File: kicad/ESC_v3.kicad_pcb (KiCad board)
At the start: 6 copper layers, 50 x 50 mm, 165 parts, among them J1 Conn_01x05_Pin, J2 Conn_01x05_Pin, J4 Conn_01x06_Pin, J6 Conn_01x06_Pin, J7 Conn_01x02_Pin, J8 Conn_01x04_Pin, J9 Conn_01x02_Pin, Q1 RH6L040BGTB1, Q10 RH6L040BGTB1, Q11 RH6L040BGTB1, Q12 RH6L040BGTB1, Q2 RH6L040BGTB1, Q3 RH6L040BGTB1, Q4 RH6L040BGTB1, Q5 RH6L040BGTB1, Q6 RH6L040BGTB1, Q7 RH6L040BGTB1, Q8 RH6L040BGTB1, Q9 RH6L040BGTB1, SW2 SW_Nidec_CAS-120A1, U1 L6387, U10 BD4104, U11 AMS1117-5.0, U12 ACS711xEXLT-15AB, U13 LM2937xMP, U14 MCP9700x-ETT, U15 MAX40200AUK, U16 AS5048A, U19 STM32G431CBUx, U2 L6387, U3 L6387, U4 L6387, U5 L6387, U6 L6387, U7 AMS1117-3.3, U8 ACS711xEXLT-15AB, U9 ACS711xEXLT-15AB

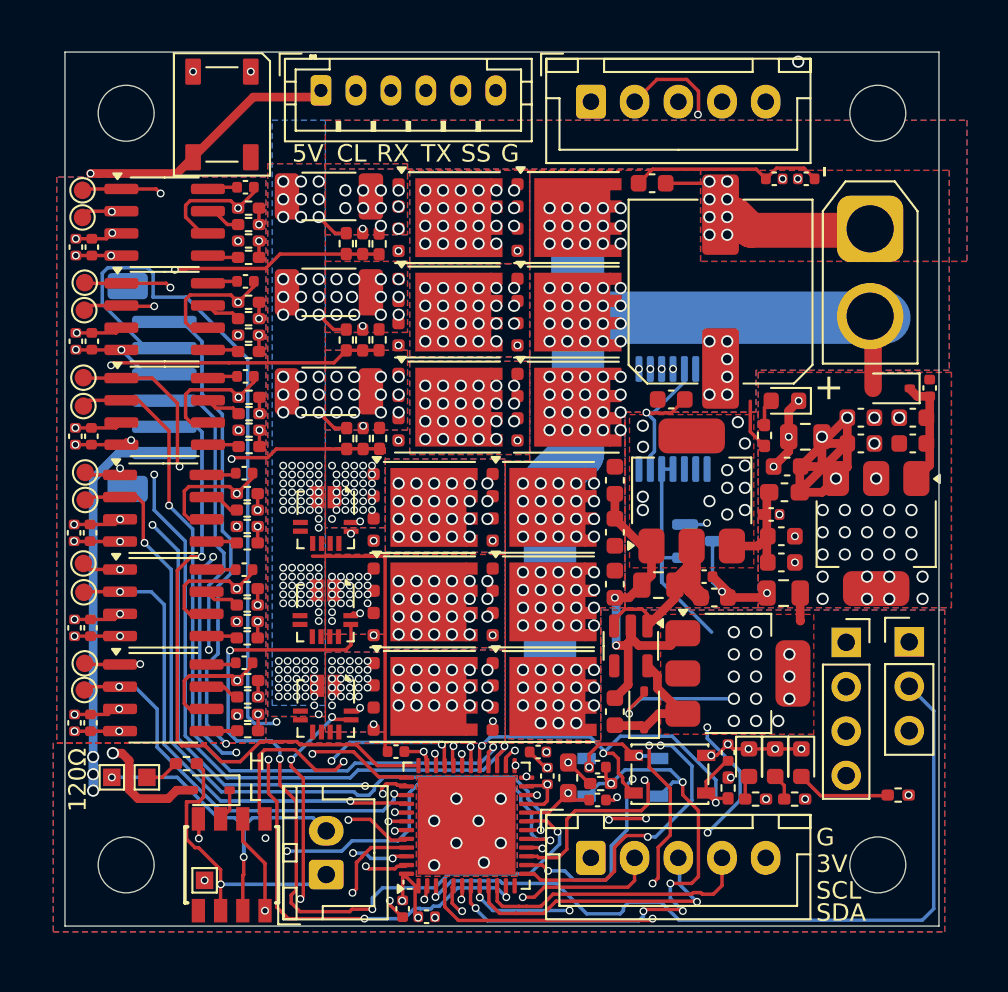
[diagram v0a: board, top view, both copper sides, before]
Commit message: a
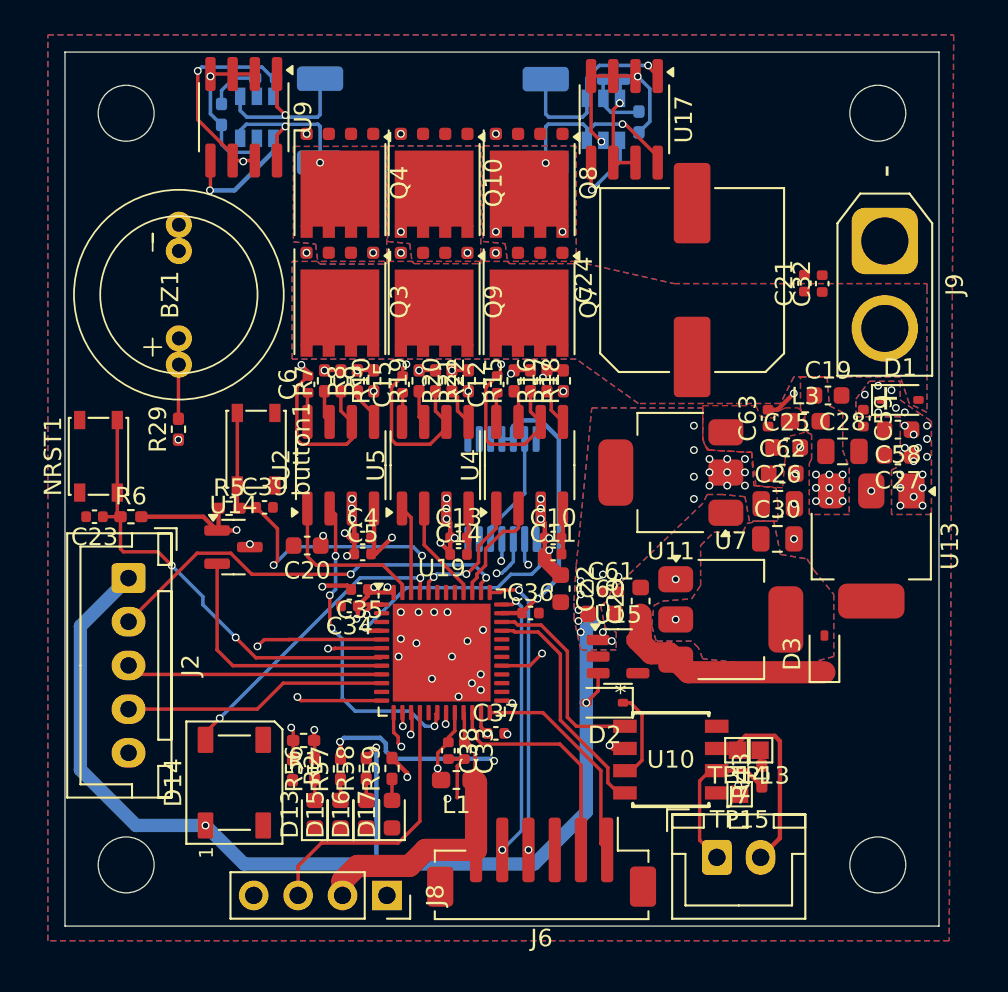
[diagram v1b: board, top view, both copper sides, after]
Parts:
- removed C1, C16, C18, C3, C7, C9: 0.1u, Capacitor_SMD:C_0402_1005Metric
- removed C17, C2, C8: 1u, Capacitor_SMD:C_0402_1005Metric
- removed C40, C41, C42, C43, C44: 22uF, Capacitor_SMD:C_0603_1608Metric
- removed G***: LOGO, agazou:full
- removed G***: LOGO, agazou:drive
- removed G***: LOGO, LOGO
- removed G***: LOGO, agazou:core
- removed G***: LOGO, agazou:blackpulsedrive
- removed J1: Conn_01x05_Pin, Connector_JST:JST_XH_B5B-XH-A_1x05_P2.50mm_Vertical
- removed J4: Conn_01x06_Pin, Connector_JST:JST_PH_B6B-PH-K_1x06_P2.00mm_Vertical
- removed Q1, Q11, Q12, Q2, Q5, Q6: RH6L040BGTB1, Package_SON:VSONP-8-1EP_5x6_P1.27mm
- removed R11, R12, R23, R24: 22, Resistor_SMD:R_0402_1005Metric_Pad0.72x0.64mm_HandSolder
- removed R13, R14, R25, R26, R3, R4: 10k, Resistor_SMD:R_0402_1005Metric_Pad0.72x0.64mm_HandSolder
- removed R44, R45, R51: 5m, Resistor_SMD:R_2010_5025Metric_Pad1.40x2.65mm_HandSolder
- removed R46, R47, R52: 1.5k, Resistor_SMD:R_0402_1005Metric_Pad0.72x0.64mm_HandSolder
- removed R48, R49, R54: 68k, Resistor_SMD:R_0402_1005Metric_Pad0.72x0.64mm_HandSolder
- removed R50, R53, R55: 2.2k, Resistor_SMD:R_0402_1005Metric_Pad0.72x0.64mm_HandSolder
- removed SW2: SW_Nidec_CAS-120A1, Connector_PinHeader_2.54mm:PinHeader_1x03_P2.54mm_Vertical
- removed TP1, TP10, TP11, TP12, TP2, TP3, TP4, TP5, TP6, TP7, TP8, TP9: TestPoint, TestPoint:TestPoint_Pad_D1.0mm
- removed U1, U3, U6: L6387, Package_SO:SOIC-8_3.9x4.9mm_P1.27mm
- added BZ1: Buzzer, jisaku:buzzer_unified, F.Cu at (56.5, 63.9)
- added R27: 2mΩ, Resistor_SMD:R_2010_5025Metric_Pad1.40x2.65mm_HandSolder, B.Cu at (64.6, 53.9)
- added R28: 2mΩ, Resistor_SMD:R_2010_5025Metric_Pad1.40x2.65mm_HandSolder, B.Cu at (77.5, 53.9)
- added R29: 100, Resistor_SMD:R_0402_1005Metric_Pad0.72x0.64mm_HandSolder, F.Cu at (56.5, 71.6)
- added R31: 100k, Resistor_SMD:R_0402_1005Metric_Pad0.72x0.64mm_HandSolder, B.Cu at (59.0, 53.6)
- added R32: 100k, Resistor_SMD:R_0402_1005Metric_Pad0.72x0.64mm_HandSolder, B.Cu at (61.5, 51.5)
- added R33: 100k, Resistor_SMD:R_0402_1005Metric_Pad0.72x0.64mm_HandSolder, B.Cu at (82.8, 54.0)
- added R34: 100k, Resistor_SMD:R_0402_1005Metric_Pad0.72x0.64mm_HandSolder, B.Cu at (81.4, 51.6)
- added U17: INA240A1D, Package_SO:SOIC-8_3.9x4.9mm_P1.27mm, F.Cu at (82.0, 53.8)
- J6, NRST1, U14: moved to F.Cu
- R1: value 22 -> 68k
- R2: value 22 -> 10k
- U12, U8: value ACS711xEXLT-15AB -> BD14210G; footprint Sensor_Current:Allegro_QFN-12-10-1EP_3x3mm_P0.5mm -> footprints:SSOP6; moved to B.Cu
- U9: value ACS711xEXLT-15AB -> INA240A1D; footprint Sensor_Current:Allegro_QFN-12-10-1EP_3x3mm_P0.5mm -> Package_SO:SOIC-8_3.9x4.9mm_P1.27mm
- moved D14 38.2 mm to (59.7, 91.8)
- moved TP14 35.8 mm to (88.5, 89.9), turned to 180 degrees
- moved D13 35.8 mm to (64.3, 93.6), turned to 90 degrees
- moved NRST1 35.2 mm to (51.9, 73.1), turned to 90 degrees
- moved J6 35.1 mm to (77.3, 96.3), turned to 180 degrees
- moved TP13 35.1 mm to (89.8, 89.9), turned to 180 degrees
- moved U8 34.0 mm to (61.0, 53.7), turned to 90 degrees
- moved R43 32.9 mm to (89.9, 91.4), turned to 90 degrees
- moved R5 32.7 mm to (59.4, 76.1), turned to 0 degrees
- moved C20 32.5 mm to (63.9, 78.2), turned to 180 degrees
- moved C23 32.1 mm to (51.7, 76.6)
- moved R56 32.0 mm to (64.3, 91.0), turned to 90 degrees
- moved TP15 31.0 mm to (88.6, 92.5), turned to 180 degrees
- moved J2 30.9 mm to (53.6, 80.1), turned to -90 degrees
- moved R6 30.9 mm to (53.8, 76.6), turned to 0 degrees
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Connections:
- Q10 pad 1: /POWER/halfHbridge8/GND_mech -> GND
- Q4 pad 1: /POWER/halfHbridge5/GND_mech -> GND
- Q8 pad 1: /POWER/halfHbridge7/GND_mech -> GND
- R1 pad 1: Net-(U1-HO) -> VCC
- R1 pad 2: Net-(Q1-G) -> ADC2_IN10
- R17 pad 1: /POWER/halfHbridge7/GND_mech -> GND
- R2 pad 1: Net-(U1-LO) -> ADC2_IN10
- R2 pad 2: Net-(Q2-G) -> GND
- R21 pad 1: /POWER/halfHbridge8/GND_mech -> GND
- R9 pad 1: /POWER/halfHbridge5/GND_mech -> GND
- U12 pad 1: /POWER/halfHbridge5/GND_mech -> ADC1_IN11
- U12 pad 3: GND -> /POWER/halfHbridge7/out1
- U12 pad 4: unconnected-(U12-~{FAULT}-Pad4) -> Net-(U12-VINM)
- U12 pad 5: unconnected-(U12-NC-Pad5) -> Net-(U12-REF)
- U12 pad 6: unconnected-(U12-NC-Pad6) -> VREF
- U4 pad 1: TIM8_CH2 -> TIM8_CH1
- U4 pad 2: TIM8_CH2N -> TIM8_CH1N
- U5 pad 1: TIM8_CH1 -> TIM8_CH2
- U5 pad 2: TIM8_CH1N -> TIM8_CH2N
- U8 pad 1: /POWER/halfHbridge8/GND_mech -> ADC2_IN12
- U8 pad 3: GND -> /POWER/halfHbridge5/out1
- U8 pad 4: unconnected-(U8-~{FAULT}-Pad4) -> Net-(U8-VINM)
- U8 pad 5: unconnected-(U8-NC-Pad5) -> Net-(U8-REF)
- U8 pad 6: unconnected-(U8-NC-Pad6) -> VREF
- U9 pad 1: /POWER/halfHbridge7/GND_mech -> Net-(U8-VINM)
- U9 pad 4: unconnected-(U9-~{FAULT}-Pad4) -> GND
- U9 pad 5: unconnected-(U9-NC-Pad5) -> ADC2_IN12
- U9 pad 6: unconnected-(U9-NC-Pad6) -> VREF
- U9 pad 7: unconnected-(U9-NC-Pad7) -> VREF
- U9 pad 8: unconnected-(U9-NC-Pad8) -> /POWER/halfHbridge5/out1
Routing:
- net +5V: track 179.3 -> 64.9 mm, vias 17 -> 24
- net OPAMP2_VINP: track 72.5 -> 0.00 mm, vias 3 -> 0
- net SS: track 85.2 -> 14.1 mm, vias 4 -> 1
- net GND: track 114.4 -> 44.3 mm, vias 194 -> 34
- net TIM3_CH1: track 65.2 -> 0.00 mm, vias 4 -> 0
- net +12V: track 139.7 -> 75.2 mm, vias 14 -> 28
- net EXTI13: track 62.1 -> 0.00 mm, vias 1 -> 0
- net OPAMP3_VINP: track 62.1 -> 0.00 mm, vias 2 -> 0
- net TIM3_CH2: track 59.0 -> 0.00 mm, vias 1 -> 0
- net TIM1_CH1: track 58.5 -> 0.00 mm, vias 2 -> 0
- net OPAMP1_VINP: track 55.7 -> 0.00 mm, vias 4 -> 0
- net TIM1_CH1N: track 54.6 -> 0.00 mm, vias 4 -> 0
- net TIM1_CH2: track 51.2 -> 0.00 mm, vias 2 -> 0
- net TIM1_CH2N: track 50.8 -> 0.00 mm, vias 3 -> 0
- net SPI1_SCK: track 68.2 -> 17.4 mm, vias 3 -> 2
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- added copper zone on In1.Cu, net +12V
- added copper zone on In4.Cu, net +12V
- added copper zone on In1.Cu, net +3.3V
- added copper zone on In4.Cu, net +3.3V
- added copper zone on In1.Cu, net +5V
- added copper zone on In4.Cu, net +5V
- added copper zone on B.Cu, net Net-(D1-K)
- added copper zone on F.Cu, net Net-(D1-K)
- added copper zone on In1.Cu, net Net-(D1-K)
- added copper zone on In2.Cu, net Net-(D1-K)
- added copper zone on In3.Cu, net Net-(D1-K)
- added copper zone on In4.Cu, net Net-(D1-K)
- added copper zone on F.Cu, net Net-(U11-VI)
- removed copper zone on B.Cu, net /POWER/halfHbridge4/GND_mech
- removed copper zone on F.Cu, net /POWER/halfHbridge4/GND_mech
- removed copper zone on In1.Cu, net /POWER/halfHbridge4/GND_mech
- removed copper zone on In2.Cu, net /POWER/halfHbridge4/GND_mech
- removed copper zone on In3.Cu, net /POWER/halfHbridge4/GND_mech
- removed copper zone on In4.Cu, net /POWER/halfHbridge4/GND_mech
- removed copper zone on B.Cu, net /POWER/halfHbridge4/out1
- removed copper zone on F.Cu, net /POWER/halfHbridge4/out1
- removed copper zone on In1.Cu, net /POWER/halfHbridge4/out1
- removed copper zone on In2.Cu, net /POWER/halfHbridge4/out1
- removed copper zone on In3.Cu, net /POWER/halfHbridge4/out1
- removed copper zone on In4.Cu, net /POWER/halfHbridge4/out1
- removed copper zone on B.Cu, net /POWER/halfHbridge5/GND_mech
- removed copper zone on F.Cu, net /POWER/halfHbridge5/GND_mech
- removed copper zone on In1.Cu, net /POWER/halfHbridge5/GND_mech
- removed copper zone on In2.Cu, net /POWER/halfHbridge5/GND_mech
- removed copper zone on In3.Cu, net /POWER/halfHbridge5/GND_mech
- removed copper zone on In4.Cu, net /POWER/halfHbridge5/GND_mech
- removed copper zone on B.Cu, net /POWER/halfHbridge6/GND_mech
- removed copper zone on F.Cu, net /POWER/halfHbridge6/GND_mech
- removed copper zone on In1.Cu, net /POWER/halfHbridge6/GND_mech
- removed copper zone on In2.Cu, net /POWER/halfHbridge6/GND_mech
- removed copper zone on In3.Cu, net /POWER/halfHbridge6/GND_mech
- removed copper zone on In4.Cu, net /POWER/halfHbridge6/GND_mech
- removed copper zone on B.Cu, net /POWER/halfHbridge6/out1
- removed copper zone on F.Cu, net /POWER/halfHbridge6/out1
- removed copper zone on In1.Cu, net /POWER/halfHbridge6/out1
- removed copper zone on In2.Cu, net /POWER/halfHbridge6/out1
- removed copper zone on In3.Cu, net /POWER/halfHbridge6/out1
- removed copper zone on In4.Cu, net /POWER/halfHbridge6/out1
- removed copper zone on B.Cu, net /POWER/halfHbridge7/GND_mech
- removed copper zone on F.Cu, net /POWER/halfHbridge7/GND_mech
- removed copper zone on In1.Cu, net /POWER/halfHbridge7/GND_mech
- removed copper zone on In2.Cu, net /POWER/halfHbridge7/GND_mech
- removed copper zone on In3.Cu, net /POWER/halfHbridge7/GND_mech
- removed copper zone on In4.Cu, net /POWER/halfHbridge7/GND_mech
- removed copper zone on B.Cu, net /POWER/halfHbridge8/GND_mech
- removed copper zone on F.Cu, net /POWER/halfHbridge8/GND_mech
- removed copper zone on In1.Cu, net /POWER/halfHbridge8/GND_mech
- removed copper zone on In2.Cu, net /POWER/halfHbridge8/GND_mech
- removed copper zone on In3.Cu, net /POWER/halfHbridge8/GND_mech
- removed copper zone on In4.Cu, net /POWER/halfHbridge8/GND_mech
- removed copper zone on B.Cu, net /POWER/halfHbridge9/GND_mech
- removed copper zone on F.Cu, net /POWER/halfHbridge9/GND_mech
- removed copper zone on In1.Cu, net /POWER/halfHbridge9/GND_mech
- removed copper zone on In2.Cu, net /POWER/halfHbridge9/GND_mech
- removed copper zone on In3.Cu, net /POWER/halfHbridge9/GND_mech
- removed copper zone on In4.Cu, net /POWER/halfHbridge9/GND_mech
- removed copper zone on B.Cu, net /POWER/halfHbridge9/out1
- removed copper zone on F.Cu, net /POWER/halfHbridge9/out1
- removed copper zone on In1.Cu, net /POWER/halfHbridge9/out1
- removed copper zone on In2.Cu, net /POWER/halfHbridge9/out1
- removed copper zone on In3.Cu, net /POWER/halfHbridge9/out1
- removed copper zone on In4.Cu, net /POWER/halfHbridge9/out1
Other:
- board text removed: "1"
- board text removed: "120Ω"
- board text removed: "2"
- board text removed: "3"
- board text removed: "3V"
- board text removed: "5V"
- board text removed: "CL"
- board text removed: "CLK"
- board text removed: "DIO"
- board text removed: "G"
- board text removed: "H"
- board text removed: "L"
- board text removed: "RST"
- board text removed: "RX"
- board text removed: "SCL"
- board text removed: "SDA"
- board text removed: "SS"
- board text removed: "TX"
